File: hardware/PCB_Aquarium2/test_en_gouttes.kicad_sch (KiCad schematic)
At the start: 24 parts, among them J10 Conn_01x03, J11 Conn_01x03, J12 Conn_01x03, J13 Conn_01x03, J14 Conn_01x03, J15 Conn_01x03, J16 Conn_01x03, J17 Conn_01x03, J18 Conn_01x03, J19 Conn_01x03, J20 Conn_01x03, J9 Conn_01x03

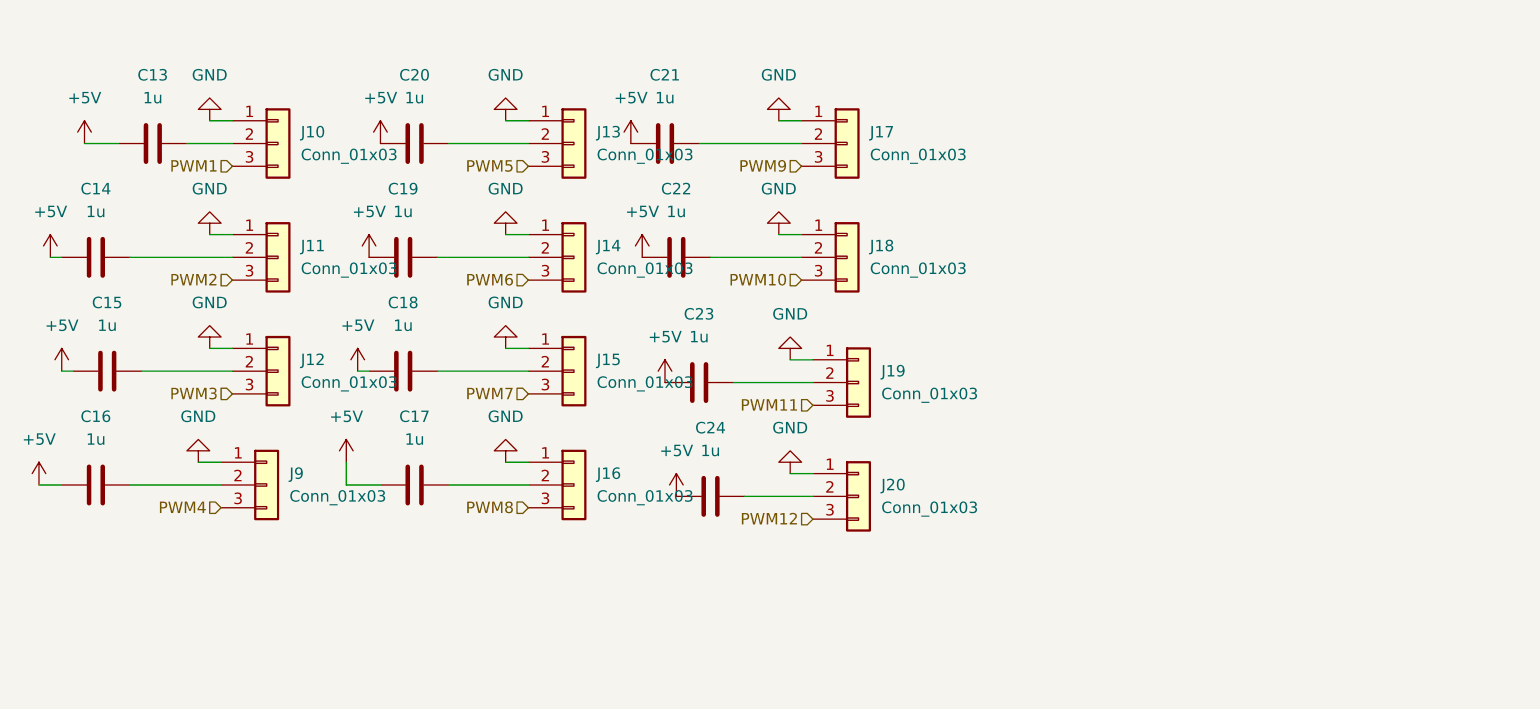
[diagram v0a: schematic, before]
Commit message: PCBs v4
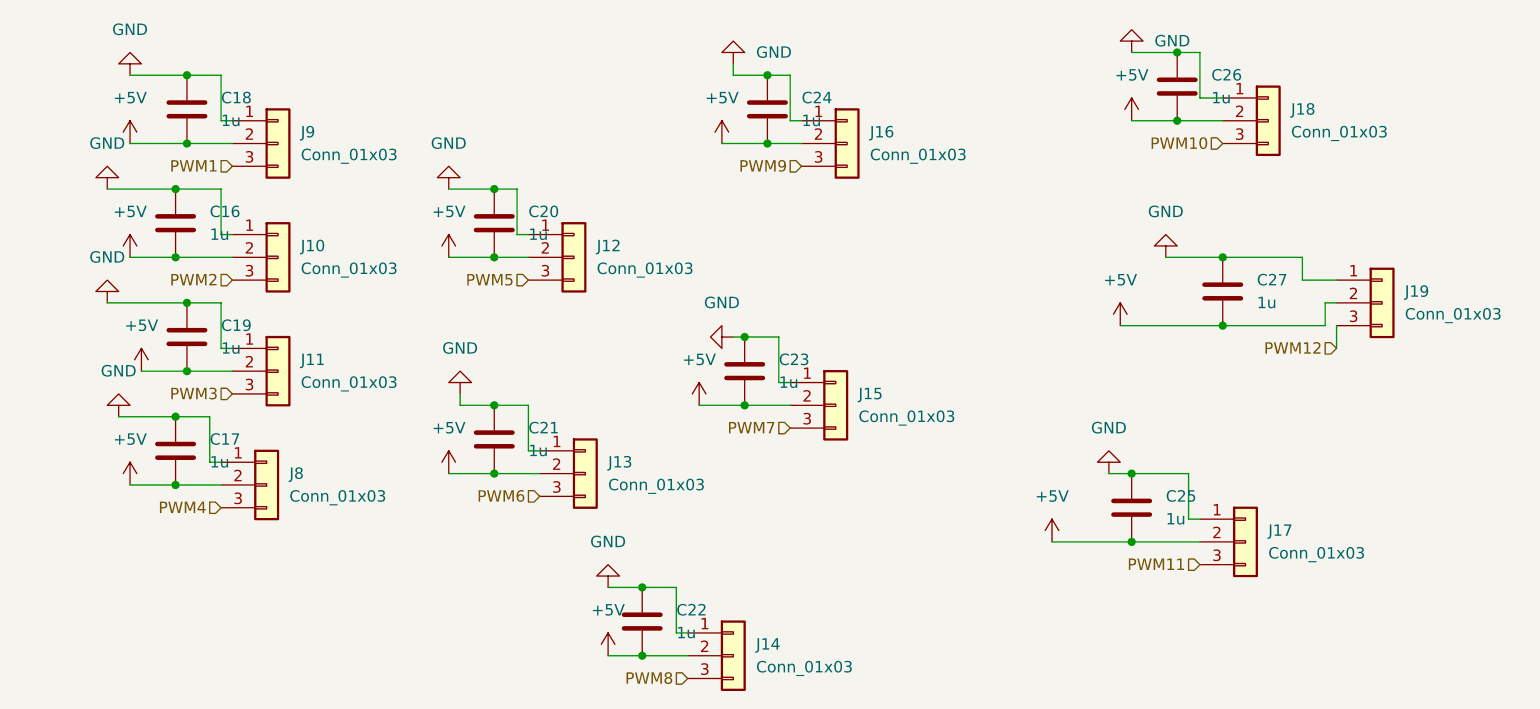
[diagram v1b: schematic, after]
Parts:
- removed C13, C14, C15: 1u, Capacitor_SMD:C_0603_1608Metric, symbol Device:C
- added C21, C22, C23: 1u, Capacitor_SMD:C_0603_1608Metric, symbol Device:C
- renumbered C21 to C24, C23 to C25, C22 to C26, C24 to C27, J11 to J10, J12 to J11, J13 to J12, J14 to J13, J16 to J14, J17 to J16, J19 to J17, J20 to J19, J9 to J8, J10 to J9
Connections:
- net +5V: now also C25.2, C26.2, J10.2 (Pin_2), J11.2 (Pin_2), J12.2 (Pin_2), J13.2 (Pin_2), J14.2 (Pin_2), J15.2 (Pin_2), J16.2 (Pin_2), J17.2 (Pin_2), J18.2 (Pin_2), J19.2 (Pin_2), J8.2 (Pin_2), J9.2 (Pin_2), C21.1, C22.1, C23.1; no longer C25.1, C26.1
- net GND: now also C16.2, C17.2, C18.2, C19.2, C20.2, C24.2, C25.1, C26.1, C27.2, C21.2, C22.2, C23.2
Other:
- moved on the sheet: C24, C25, C26, C27, J12, J13, J14, J15, J17, J18, J19
